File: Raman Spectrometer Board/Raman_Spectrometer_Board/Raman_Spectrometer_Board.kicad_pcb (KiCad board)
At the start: 2 copper layers, 65.5 x 91.4 mm, 37 parts, among them J1 RJ45_LED_Shielded, Q1 BSS138, Q2 BSS138, Q3 BSS138, Q4 BSS138, SW1 SW_Push, SW2 SW_Push, U1 Teensy4.1_DEV-16771, U2 OKI 12V-5V

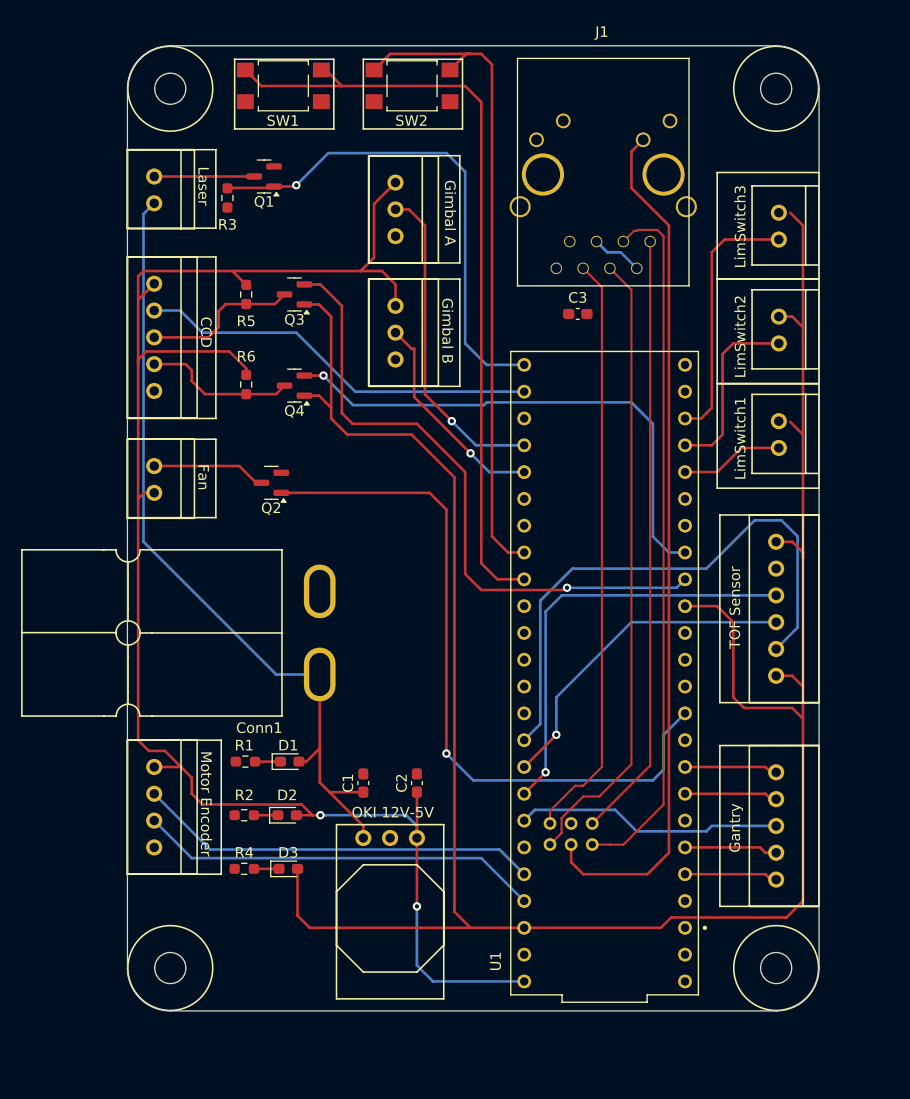
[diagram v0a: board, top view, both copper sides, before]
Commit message: Finished Rev2
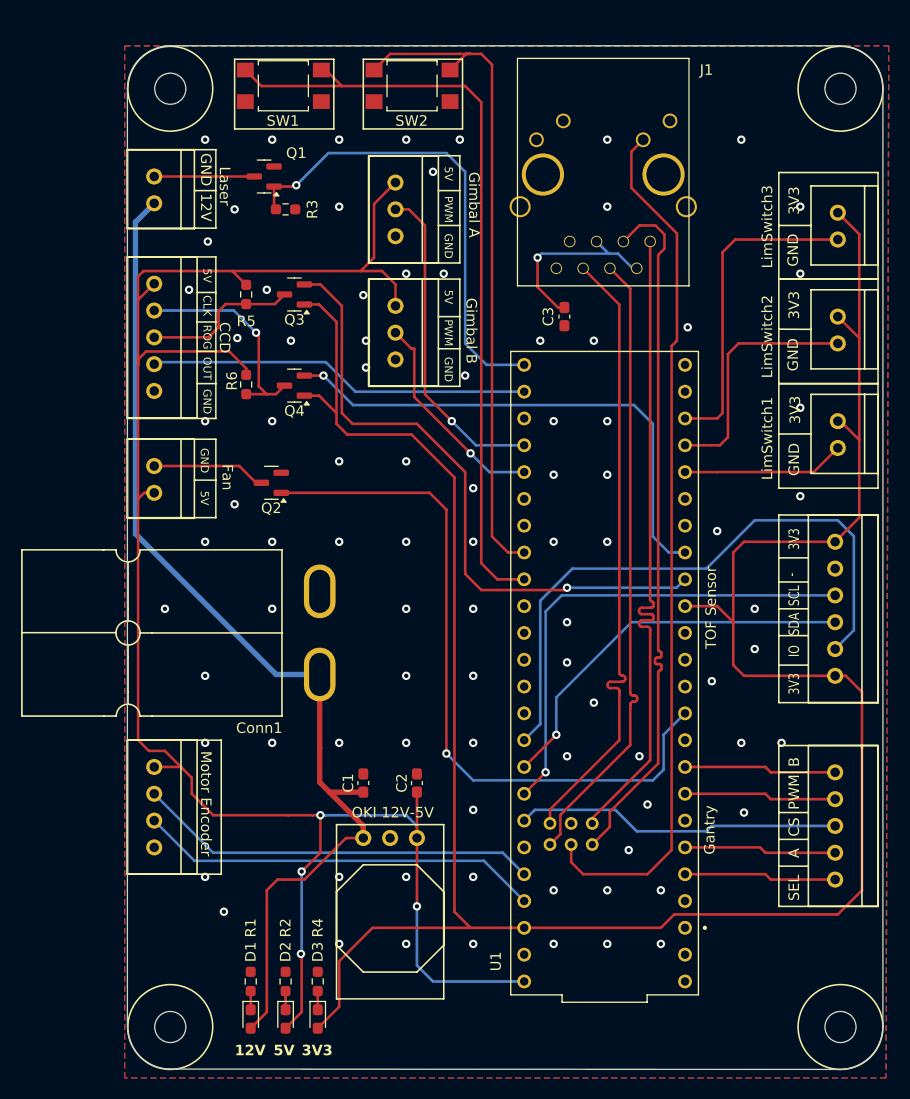
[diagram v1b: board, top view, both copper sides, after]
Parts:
- moved D1 24.7 mm to (86.9, 111.3), turned to -90 degrees
- moved R1 20.8 mm to (86.9, 107.7), turned to 90 degrees
- moved D2 19.3 mm to (90.2, 111.3), turned to -90 degrees
- moved R2 16.2 mm to (90.2, 107.7), turned to 90 degrees
- moved D3 14.5 mm to (93.2, 111.3), turned to -90 degrees
- moved R4 12.7 mm to (93.2, 107.7), turned to 90 degrees
- moved H4 8.27 mm to (142.7, 112.0), turned to 90 degrees
- moved H3 6.10 mm to (142.7, 23.1)
- moved R3 5.61 mm to (90.2, 34.5), turned to 0 degrees
- moved Conn2 5.59 mm to (142.2, 66.0)
- moved Conn6 5.59 mm to (142.2, 87.9)
- moved Conn10 5.59 mm to (142.5, 54.6)
- moved Conn8 5.59 mm to (142.5, 34.9)
- moved Conn9 5.59 mm to (142.5, 44.7)
- moved H2 5.59 mm to (79.2, 112.0)
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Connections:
- Conn5 pad 2: CCD_Vout -> CCD_CLK_5V
- Conn5 pad 4: CCD_CLK_5V -> CCD_Vout
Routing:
- net +12V: track 77.6 -> 100.3 mm
- net +5V: track 162.2 -> 182.4 mm, vias 2 -> 4
- net Net-(C3-Pad1): track 4.86 -> 18.0 mm, vias 0 -> 1
- net +3.3V: track 223.2 -> 229.9 mm
- net CCD_CLK_5V: track 14.5 -> 20.7 mm, vias 0 -> 1
- net Limit Switch 1: track 24.5 -> 30.4 mm
- net Limit Switch 2: track 17.4 -> 23.1 mm
- net SDA: track 31.6 -> 37.2 mm
- net SCL: track 40.6 -> 46.2 mm
- net PWM: track 8.85 -> 14.4 mm
- net IN_A: track 8.85 -> 14.4 mm
- net CS: track 25.3 -> 30.9 mm
- net SEL: track 8.85 -> 14.4 mm
- net IN_B: track 8.85 -> 14.4 mm
- net Limit Switch 3: track 9.84 -> 15.4 mm
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- added copper zone on B.Cu, net GND
- added copper zone on F.Cu, net GND
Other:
- board size 65.5 x 91.4 mm -> 71.6 x 97 mm
- board text added: "-"
- board text added: "12V"
- board text added: "3V3"
- board text added: "5V"
- board text added: "A"
- board text added: "B"
- board text added: "CLK"
- board text added: "CS"
- board text added: "GND"
- board text added: "IO"
- board text added: "OUT"
- board text added: "PWM"
- board text added: "ROG"
- board text added: "SCL"
- board text added: "SDA"
- board text added: "SEL"
